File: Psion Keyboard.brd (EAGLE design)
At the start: 100 x 80 mm, 3 parts, among them X2 52745-2290

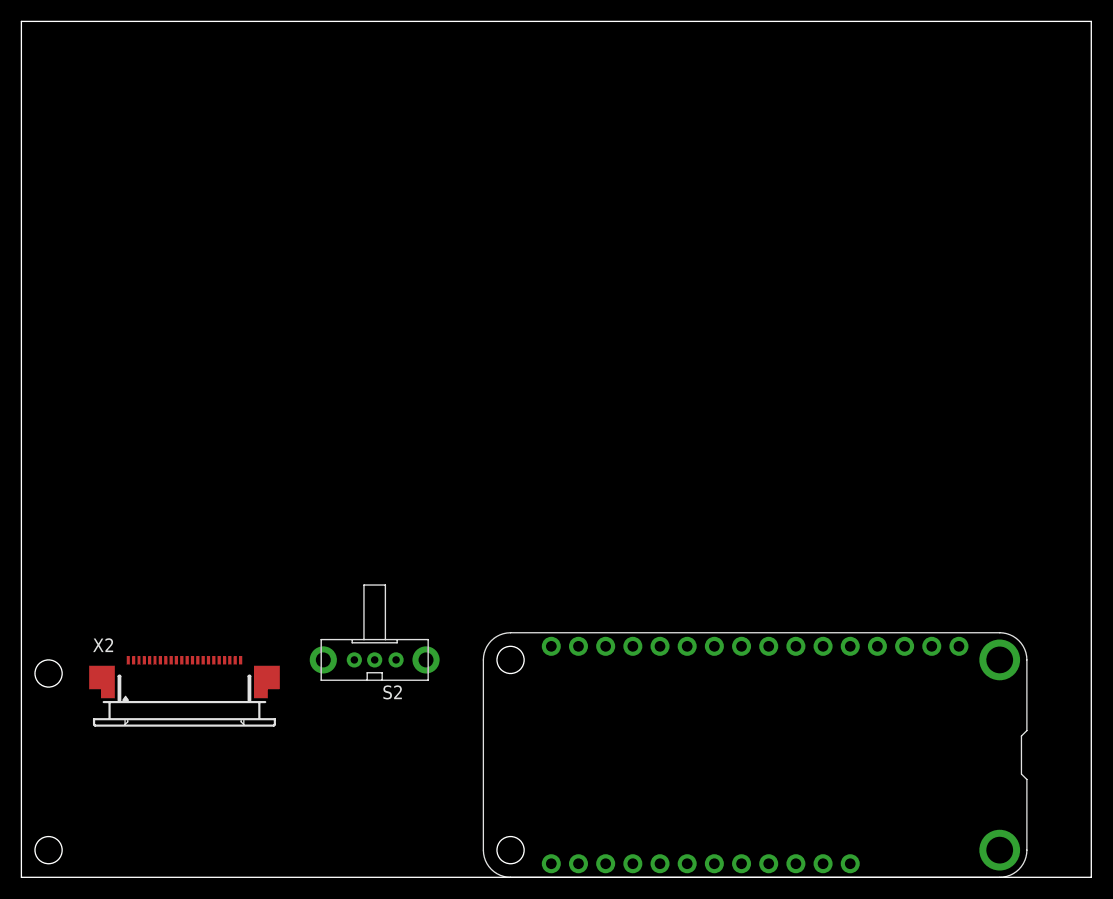
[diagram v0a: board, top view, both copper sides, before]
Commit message: Basic board shape.
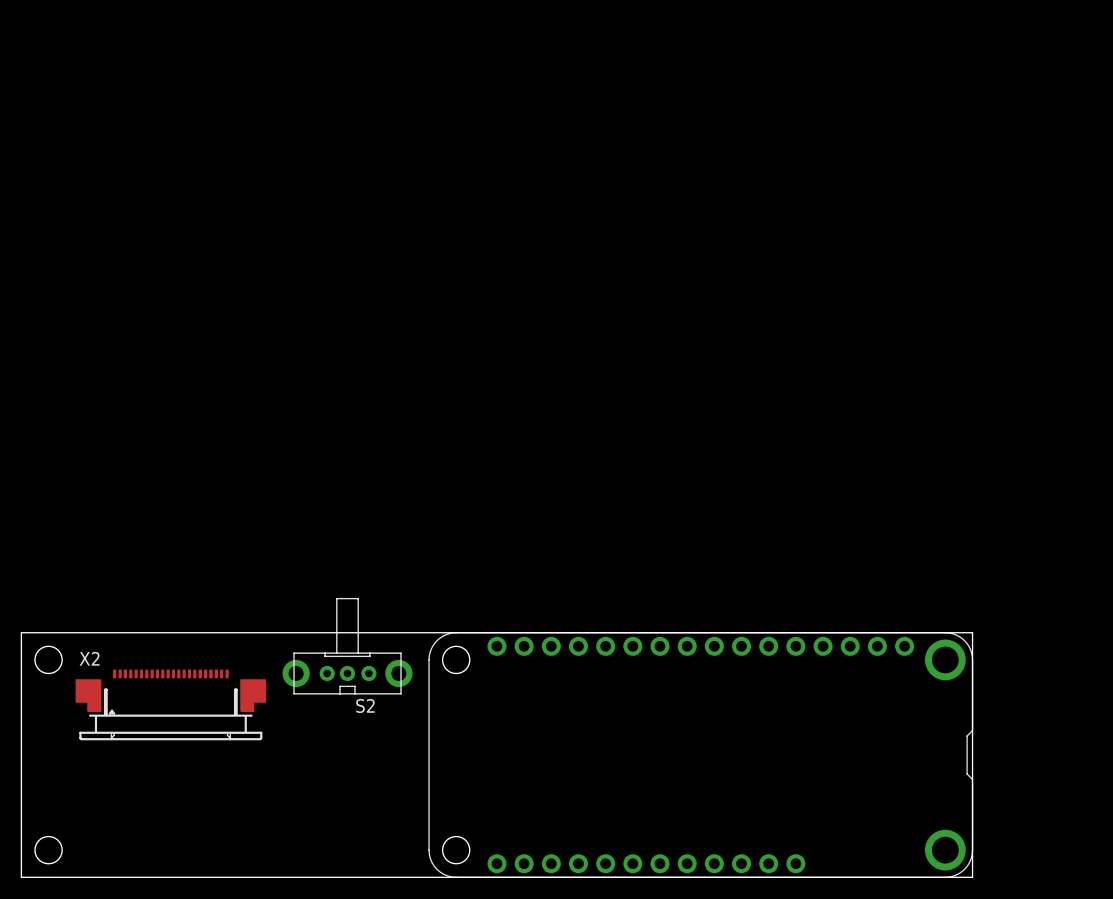
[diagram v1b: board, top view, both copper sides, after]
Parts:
- moved MS1 5.08 mm to (88.9, 22.9)
- moved S2 2.84 mm to (30.5, 19.1)
- moved X2 1.80 mm to (14.0, 16.5)
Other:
- board size 100 x 80 mm -> 88.9 x 22.9 mm
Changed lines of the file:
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@@
 <setting verticaltext="up"/>
 </settings>
-<grid distance="50" unitdist="mil" unit="mil" style="lines" multiple="1" display="yes" altdistance="5" altunitdist="mil" altunit="mil"/>
+<grid distance="50" unitdist="mil" unit="mil" style="lines" multiple="1" display="yes" altdistance="0.1" altunitdist="mil" altunit="mil"/>
 <layers>
 <layer number="1" name="Top" color="4" fill="1" visible="yes" active="yes"/>
@@
 <board>
 <plain>
-<wire x1="0" y1="0" x2="100" y2="0" width="0" layer="20"/>
-<wire x1="100" y1="0" x2="100" y2="80" width="0" layer="20"/>
-<wire x1="100" y1="80" x2="0" y2="80" width="0" layer="20"/>
-<wire x1="0" y1="80" x2="0" y2="0" width="0" layer="20"/>
+<wire x1="0" y1="0" x2="88.9002" y2="0" width="0" layer="20"/>
+<wire x1="88.9002" y1="0" x2="88.900196875" y2="22.860159375" width="0" layer="20"/>
+<wire x1="88.900196875" y1="22.860159375" x2="0" y2="22.860159375" width="0" layer="20"/>
+<wire x1="0" y1="22.860159375" x2="0" y2="0" width="0" layer="20"/>
 <circle x="2.54" y="2.54" radius="1.27" width="0.000025" layer="20"/>
-<circle x="2.54" y="19.05" radius="1.27" width="0.000025" layer="20"/>
+<circle x="2.54" y="20.32" radius="1.27" width="0.000025" layer="20"/>
 </plain>
 <attributes>
@@
 </autorouter>
 <elements>
-<element name="MS1" library="adafruit" library_urn="urn:adsk.eagle:library:420" package="FEATHERWING_DIM" value="FEATHERWING_NODIM" x="93.98" y="22.86" rot="R180"/>
-<element name="S2" library="adafruit" library_urn="urn:adsk.eagle:library:420" package="EG1213" value="EG1213" x="33.02" y="20.32" rot="R180"/>
-<element name="X2" library="con-molex" library_urn="urn:adsk.eagle:library:165" package="52745-2290" value="52745-2290" x="15.24" y="17.78">
-<attribute name="MF" value="MOLEX" x="15.24" y="17.78" size="1.778" layer="27" display="off"/>
-<attribute name="MPN" value="" x="15.24" y="17.78" size="1.778" layer="27" display="off"/>
-<attribute name="OC_FARNELL" value="unknown" x="15.24" y="17.78" size="1.778" layer="27" display="off"/>
-<attribute name="OC_NEWARK" value="unknown" x="15.24" y="17.78" size="1.778" layer="27" display="off"/>
+<element name="MS1" library="adafruit" library_urn="urn:adsk.eagle:library:420" package="FEATHERWING_DIM" value="FEATHERWING_NODIM" x="88.9" y="22.86" rot="R180"/>
+<element name="S2" library="adafruit" library_urn="urn:adsk.eagle:library:420" package="EG1213" value="EG1213" x="30.48" y="19.05" rot="R180"/>
+<element name="X2" library="con-molex" library_urn="urn:adsk.eagle:library:165" package="52745-2290" value="52745-2290" x="13.97" y="16.51">
+<attribute name="MF" value="MOLEX" x="13.97" y="16.51" size="1.778" layer="27" display="off"/>
+<attribute name="MPN" value="" x="13.97" y="16.51" size="1.778" layer="27" display="off"/>
+<attribute name="OC_FARNELL" value="unknown" x="13.97" y="16.51" size="1.778" layer="27" display="off"/>
+<attribute name="OC_NEWARK" value="unknown" x="13.97" y="16.51" size="1.778" layer="27" display="off"/>
 </element>
 </elements>
@@
 <contactref element="S2" pad="1"/>
 <contactref element="MS1" pad="4"/>
-<wire x1="35.02" y1="20.32" x2="80.01" y2="21.59" width="0" layer="19" extent="1-1"/>
+<wire x1="32.48" y1="19.05" x2="74.93" y2="21.59" width="0" layer="19" extent="1-1"/>
 </signal>
 <signal name="EN">
 <contactref element="S2" pad="2"/>
 <contactref element="MS1" pad="27"/>
-<wire x1="33.02" y1="20.32" x2="74.93" y2="1.27" width="0" layer="19" extent="1-1"/>
+<wire x1="30.48" y1="19.05" x2="69.85" y2="1.27" width="0" layer="19" extent="1-1"/>
 </signal>
 <signal name="SDA">
@@
 <contactref element="X2" pad="2"/>
 <contactref element="X2" pad="5"/>
-<wire x1="11.99" y1="20.28" x2="10.49" y2="20.28" width="0" layer="19" extent="1-1"/>
-<wire x1="49.53" y1="1.27" x2="11.99" y2="20.28" width="0" layer="19" extent="1-1"/>
+<wire x1="10.72" y1="19.01" x2="9.22" y2="19.01" width="0" layer="19" extent="1-1"/>
+<wire x1="44.45" y1="1.27" x2="10.72" y2="19.01" width="0" layer="19" extent="1-1"/>
 </signal>
 <signal name="SCL">
 <contactref element="MS1" pad="18"/>
 <contactref element="X2" pad="3"/>
-<wire x1="52.07" y1="1.27" x2="10.99" y2="20.28" width="0" layer="19" extent="1-1"/>
+<wire x1="46.99" y1="1.27" x2="9.72" y2="19.01" width="0" layer="19" extent="1-1"/>
 </signal>
 <signal name="27">
 <contactref element="MS1" pad="19"/>
 <contactref element="X2" pad="4"/>
-<wire x1="54.61" y1="1.27" x2="11.49" y2="20.28" width="0" layer="19" extent="1-1"/>
+<wire x1="49.53" y1="1.27" x2="10.22" y2="19.01" width="0" layer="19" extent="1-1"/>
 </signal>
 <signal name="30">
 <contactref element="MS1" pad="20"/>
 <contactref element="X2" pad="6"/>
-<wire x1="57.15" y1="1.27" x2="12.49" y2="20.28" width="0" layer="19" extent="1-1"/>
+<wire x1="52.07" y1="1.27" x2="11.22" y2="19.01" width="0" layer="19" extent="1-1"/>
 </signal>
 <signal name="11">
 <contactref element="MS1" pad="22"/>
 <contactref element="X2" pad="7"/>
-<wire x1="12.99" y1="20.28" x2="62.23" y2="1.27" width="0" layer="19" extent="1-1"/>
+<wire x1="11.72" y1="19.01" x2="57.15" y2="1.27" width="0" layer="19" extent="1-1"/>
 </signal>
 <signal name="7">
 <contactref element="MS1" pad="23"/>
 <contactref element="X2" pad="8"/>
-<wire x1="13.49" y1="20.28" x2="64.77" y2="1.27" width="0" layer="19" extent="1-1"/>
+<wire x1="12.22" y1="19.01" x2="59.69" y2="1.27" width="0" layer="19" extent="1-1"/>
 </signal>
 <signal name="15">
 <contactref element="MS1" pad="24"/>
 <contactref element="X2" pad="9"/>
-<wire x1="13.99" y1="20.28" x2="67.31" y2="1.27" width="0" layer="19" extent="1-1"/>
+<wire x1="12.72" y1="19.01" x2="62.23" y2="1.27" width="0" layer="19" extent="1-1"/>
 </signal>
 <signal name="16">
 <contactref element="MS1" pad="25"/>
 <contactref element="X2" pad="10"/>
-<wire x1="14.49" y1="20.28" x2="69.85" y2="1.27" width="0" layer="19" extent="1-1"/>
+<wire x1="13.22" y1="19.01" x2="64.77" y2="1.27" width="0" layer="19" extent="1-1"/>
 </signal>
 <signal name="USB">
@@
 <contactref element="MS1" pad="15"/>
 <contactref element="X2" pad="21"/>
-<wire x1="19.99" y1="20.28" x2="52.07" y2="21.59" width="0" layer="19" extent="1-1"/>
+<wire x1="18.72" y1="19.01" x2="46.99" y2="21.59" width="0" layer="19" extent="1-1"/>
 </signal>
 <signal name="RXD">
 <contactref element="MS1" pad="14"/>
 <contactref element="X2" pad="20"/>
-<wire x1="19.49" y1="20.28" x2="54.61" y2="21.59" width="0" layer="19" extent="1-1"/>
+<wire x1="18.22" y1="19.01" x2="49.53" y2="21.59" width="0" layer="19" extent="1-1"/>
 </signal>
 <signal name="MISO">
 <contactref element="MS1" pad="13"/>
 <contactref element="X2" pad="19"/>
-<wire x1="18.99" y1="20.28" x2="57.15" y2="21.59" width="0" layer="19" extent="1-1"/>
+<wire x1="17.72" y1="19.01" x2="52.07" y2="21.59" width="0" layer="19" extent="1-1"/>
 </signal>
 <signal name="MOSI">
 <contactref element="MS1" pad="12"/>
 <contactref element="X2" pad="18"/>
-<wire x1="18.49" y1="20.28" x2="59.69" y2="21.59" width="0" layer="19" extent="1-1"/>
+<wire x1="17.22" y1="19.01" x2="54.61" y2="21.59" width="0" layer="19" extent="1-1"/>
 </signal>
 <signal name="SCK">
 <contactref element="MS1" pad="11"/>
 <contactref element="X2" pad="17"/>
-<wire x1="17.99" y1="20.28" x2="62.23" y2="21.59" width="0" layer="19" extent="1-1"/>
+<wire x1="16.72" y1="19.01" x2="57.15" y2="21.59" width="0" layer="19" extent="1-1"/>
 </signal>
 <signal name="A5">
 <contactref element="MS1" pad="10"/>
 <contactref element="X2" pad="16"/>
-<wire x1="17.49" y1="20.28" x2="64.77" y2="21.59" width="0" layer="19" extent="1-1"/>
+<wire x1="16.22" y1="19.01" x2="59.69" y2="21.59" width="0" layer="19" extent="1-1"/>
 </signal>
 <signal name="A4">
 <contactref element="MS1" pad="9"/>
 <contactref element="X2" pad="15"/>
-<wire x1="16.99" y1="20.28" x2="67.31" y2="21.59" width="0" layer="19" extent="1-1"/>
+<wire x1="15.72" y1="19.01" x2="62.23" y2="21.59" width="0" layer="19" extent="1-1"/>
 </signal>
 <signal name="A3">
 <contactref element="MS1" pad="8"/>
 <contactref element="X2" pad="14"/>
-<wire x1="16.49" y1="20.28" x2="69.85" y2="21.59" width="0" layer="19" extent="1-1"/>
+<wire x1="15.22" y1="19.01" x2="64.77" y2="21.59" width="0" layer="19" extent="1-1"/>
 </signal>
 <signal name="A2">
 <contactref element="MS1" pad="7"/>
 <contactref element="X2" pad="13"/>
-<wire x1="15.99" y1="20.28" x2="72.39" y2="21.59" width="0" layer="19" extent="1-1"/>
+<wire x1="14.72" y1="19.01" x2="67.31" y2="21.59" width="0" layer="19" extent="1-1"/>
 </signal>
 <signal name="A1">
 <contactref element="MS1" pad="6"/>
 <contactref element="X2" pad="12"/>
-<wire x1="15.49" y1="20.28" x2="74.93" y2="21.59" width="0" layer="19" extent="1-1"/>
+<wire x1="14.22" y1="19.01" x2="69.85" y2="21.59" width="0" layer="19" extent="1-1"/>
 </signal>
 <signal name="A0">
 <contactref element="MS1" pad="5"/>
 <contactref element="X2" pad="11"/>
-<wire x1="14.99" y1="20.28" x2="77.47" y2="21.59" width="0" layer="19" extent="1-1"/>
+<wire x1="13.72" y1="19.01" x2="72.39" y2="21.59" width="0" layer="19" extent="1-1"/>
 </signal>
 </signals>
